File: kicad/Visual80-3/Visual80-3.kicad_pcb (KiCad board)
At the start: 2 copper layers, 18.4 x 59.1 mm, 6 parts, among them J1 PMOD, U1 Z80, U3 74HCT02, U4 74HCT574

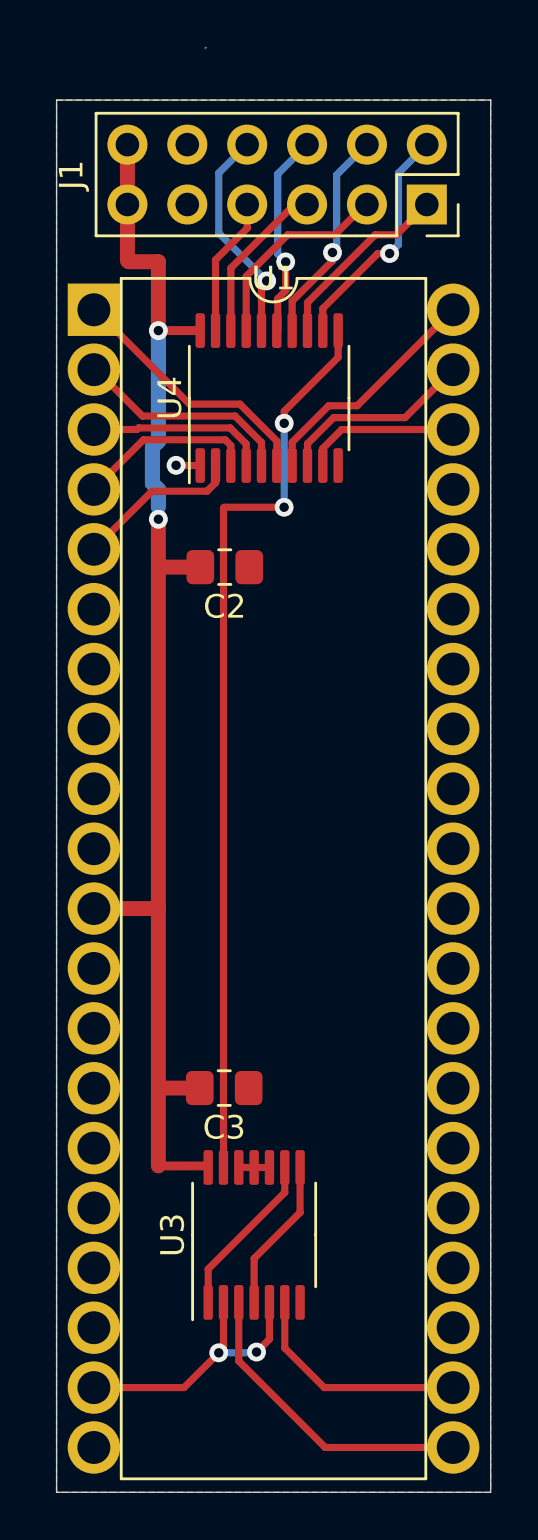
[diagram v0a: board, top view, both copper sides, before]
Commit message: Added dislay PCB design.  Added pictures.  Updated readme.
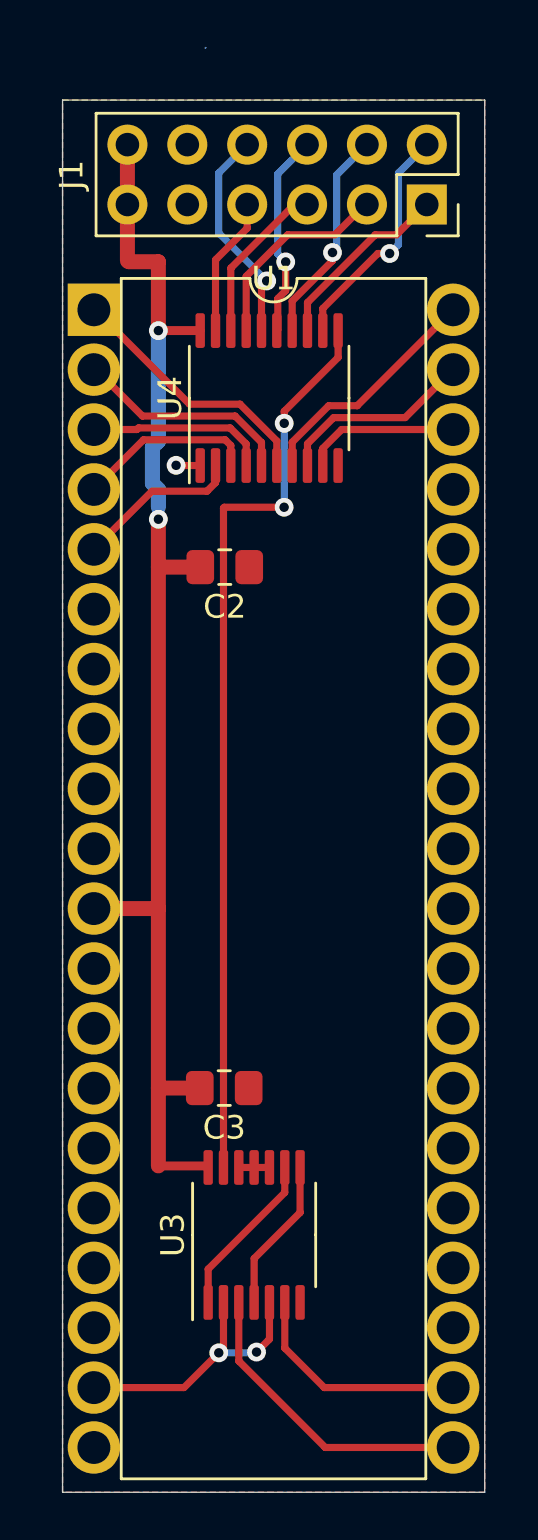
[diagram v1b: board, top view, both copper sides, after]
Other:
- board size 18.4 x 59.1 mm -> 17.9 x 59.1 mm
